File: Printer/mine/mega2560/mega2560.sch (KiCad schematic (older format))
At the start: 1 part

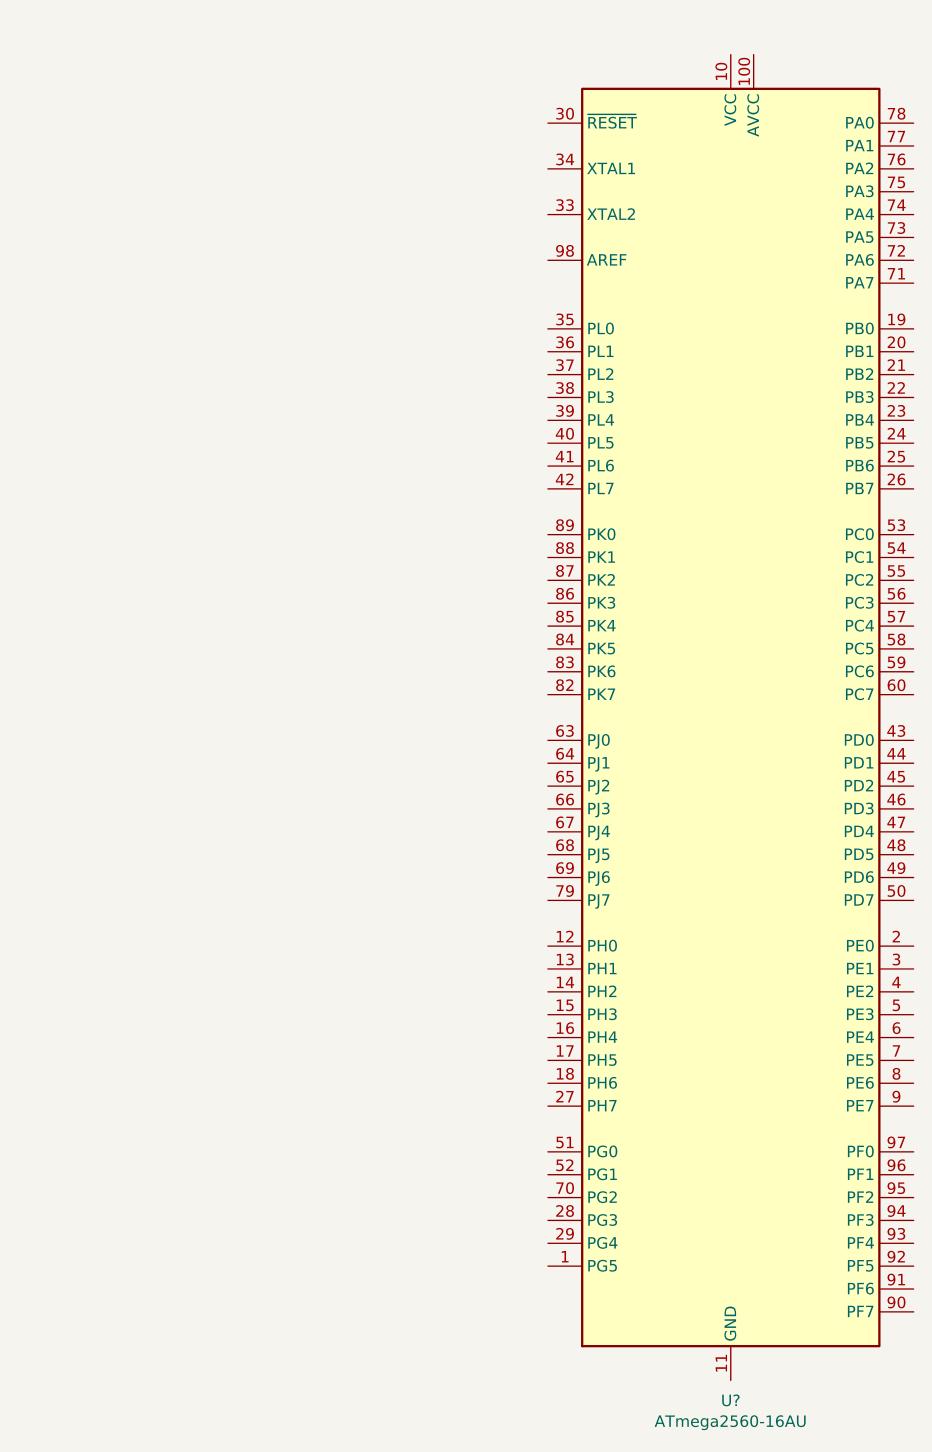
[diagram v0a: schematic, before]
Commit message: f
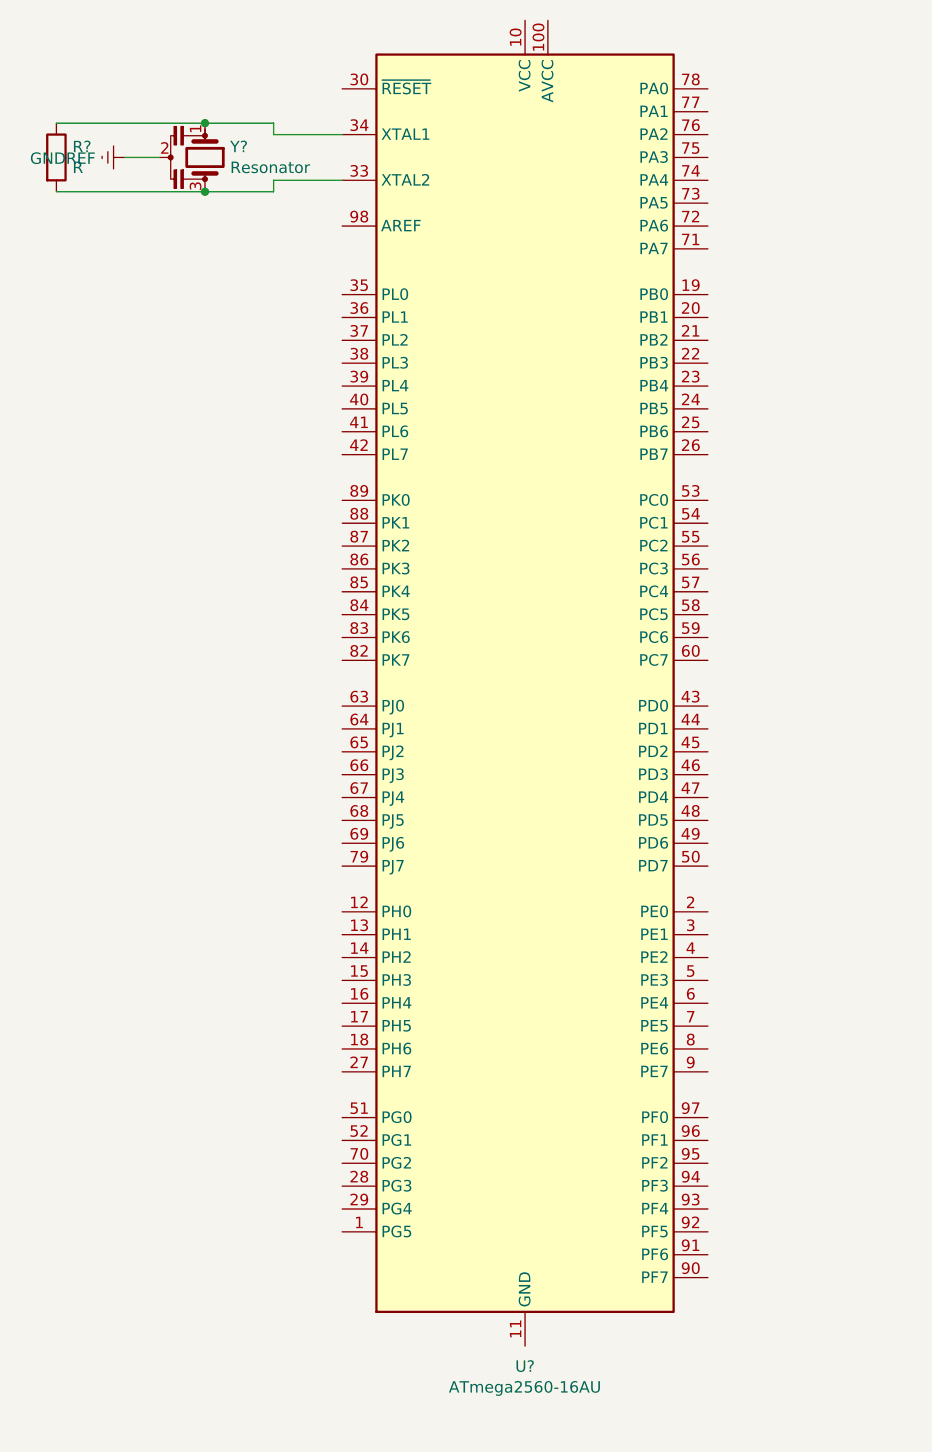
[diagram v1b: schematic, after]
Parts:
- removed U?: ATmega2560-16AU, Package_QFP:TQFP-100_14x14mm_P0.5mm, symbol MCU_Microchip_ATmega:ATmega2560-16AU
- added R?: R, symbol Device:R
- added U?: ATmega2560-16AU, Package_QFP:TQFP-100_14x14mm_P0.5mm, symbol MCU_Microchip_ATmega:ATmega2560-16AU
- added Y?: Resonator, symbol Device:Resonator
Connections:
- new net: U?.10 (VCC), U?.31 (VCC), U?.61 (VCC), U?.80 (VCC)
- new net: U?.11 (GND), U?.32 (GND), U?.62 (GND), U?.81 (GND), U?.99 (GND)
- new net: R?.2, U?.33 (XTAL2), Y?.3
- new net: R?.1, U?.34 (XTAL1), Y?.1
- new net GNDREF: Y?.2
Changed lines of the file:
@@
 EELAYER 30 0
 EELAYER END
-$Descr A4 11693 8268
+$Descr A3 16535 11693
 encoding utf-8
 Sheet 1 1
@@
 $Comp
 L MCU_Microchip_ATmega:ATmega2560-16AU U?
-U 1 1 61C9711E
-P 4000 4000
-F 0 "U?" H 4000 1011 50  0000 C CNN
-F 1 "ATmega2560-16AU" H 4000 920 50  0000 C CNN
-F 2 "Package_QFP:TQFP-100_14x14mm_P0.5mm" H 4000 4000 50  0001 C CIN
-F 3 "http://ww1.microchip.com/downloads/en/DeviceDoc/Atmel-2549-8-bit-AVR-Microcontroller-ATmega640-1280-1281-2560-2561_datasheet.pdf" H 4000 4000 50  0001 C CNN
-	1    4000 4000
+U 1 1 61CC0B3F
+P 3100 3850
+F 0 "U?" H 3100 861 50  0000 C CNN
+F 1 "ATmega2560-16AU" H 3100 770 50  0000 C CNN
+F 2 "Package_QFP:TQFP-100_14x14mm_P0.5mm" H 3100 3850 50  0001 C CIN
+F 3 "http://ww1.microchip.com/downloads/en/DeviceDoc/Atmel-2549-8-bit-AVR-Microcontroller-ATmega640-1280-1281-2560-2561_datasheet.pdf" H 3100 3850 50  0001 C CNN
+	1    3100 3850
 	1    0    0    -1
 $EndComp
+$Comp
+L Device:Resonator Y?
+U 1 1 61CCCFDC
+P 1700 1550
+F 0 "Y?" V 1654 1660 50  0000 L CNN
+F 1 "Resonator" V 1745 1660 50  0000 L CNN
+F 2 "" H 1675 1550 50  0001 C CNN
+F 3 "~" H 1675 1550 50  0001 C CNN
+	1    1700 1550
+	0    1    1    0
+$EndComp
+Wire Wire Line
+	2300 1450 2000 1450
+Wire Wire Line
+	2000 1450 2000 1400
+Wire Wire Line
+	2000 1400 1700 1400
+Connection ~ 1700 1400
+Wire Wire Line
+	1700 1400 1050 1400
+Wire Wire Line
+	2300 1650 2000 1650
+Wire Wire Line
+	2000 1650 2000 1700
+Wire Wire Line
+	2000 1700 1700 1700
+Connection ~ 1700 1700
+Wire Wire Line
+	1700 1700 1050 1700
+$Comp
+L power:GNDREF #PWR?
+U 1 1 61CDC846
+P 1350 1550
+F 0 "#PWR?" H 1350 1300 50  0001 C CNN
+F 1 "GNDREF" V 1355 1422 50  0000 R CNN
+F 2 "" H 1350 1550 50  0001 C CNN
+F 3 "" H 1350 1550 50  0001 C CNN
+	1    1350 1550
+	0    1    1    0
+$EndComp
+Wire Wire Line
+	1500 1550 1350 1550
+$Comp
+L Device:R R?
+U 1 1 61CDDBB1
+P 1050 1550
+F 0 "R?" H 1120 1596 50  0000 L CNN
+F 1 "R" H 1120 1505 50  0000 L CNN
+F 2 "" V 980 1550 50  0001 C CNN
+F 3 "~" H 1050 1550 50  0001 C CNN
+	1    1050 1550
+	1    0    0    -1
+$EndComp
